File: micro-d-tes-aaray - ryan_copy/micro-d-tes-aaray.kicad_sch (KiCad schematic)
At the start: 23 parts, among them J22 Conn_01x01_Socket, J23 Conn_01x01_Socket, J24 Conn_01x01_Socket, J25 Conn_01x01_Socket, J26 Conn_01x01_Socket, J27 Conn_01x01_Socket, J28 Conn_01x01_Socket, J29 Conn_01x01_Socket, J30 Conn_01x01_Socket, J31 Conn_01x01_Socket, J32 Conn_01x01_Socket, J33 Conn_01x01_Socket, J34 Conn_01x01_Socket, J35 Conn_01x01_Socket, J36 Conn_01x01_Socket, J37 Conn_01x01_Socket, J38 Conn_01x01_Socket, J39 Conn_01x01_Socket, J40 Conn_01x01_Socket, J41 Conn_01x01_Socket, J42 DB25_Plug

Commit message: update
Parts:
- H3, H4: footprint 0_footprint_Library:MountingHole_3mm_4-40_DIN965_Pad -> 0_footprint_Library:MountingHole_3mm_2-56_DIN965_Pad
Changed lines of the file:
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@@
       (effects (font (size 1.27 1.27)) (justify left))
     )
-    (property "Footprint" "0_footprint_Library:MountingHole_3mm_4-40_DIN965_Pad" (at 55.88 143.51 0)
+    (property "Footprint" "0_footprint_Library:MountingHole_3mm_2-56_DIN965_Pad" (at 55.88 143.51 0)
       (effects (font (size 1.27 1.27)) hide)
     )
@@
       (effects (font (size 1.27 1.27)) (justify left))
     )
-    (property "Footprint" "0_footprint_Library:MountingHole_3mm_4-40_DIN965_Pad" (at 59.69 143.51 0)
-      (effects (font (size 1.27 1.27)) hide)
-    )
+    (property "Footprint" "0_footprint_Library:MountingHole_3mm_2-56_DIN965_Pad" (at 59.69 143.51 0)
+      (effects (font (size 1.27 1.27)) hide)
+    )

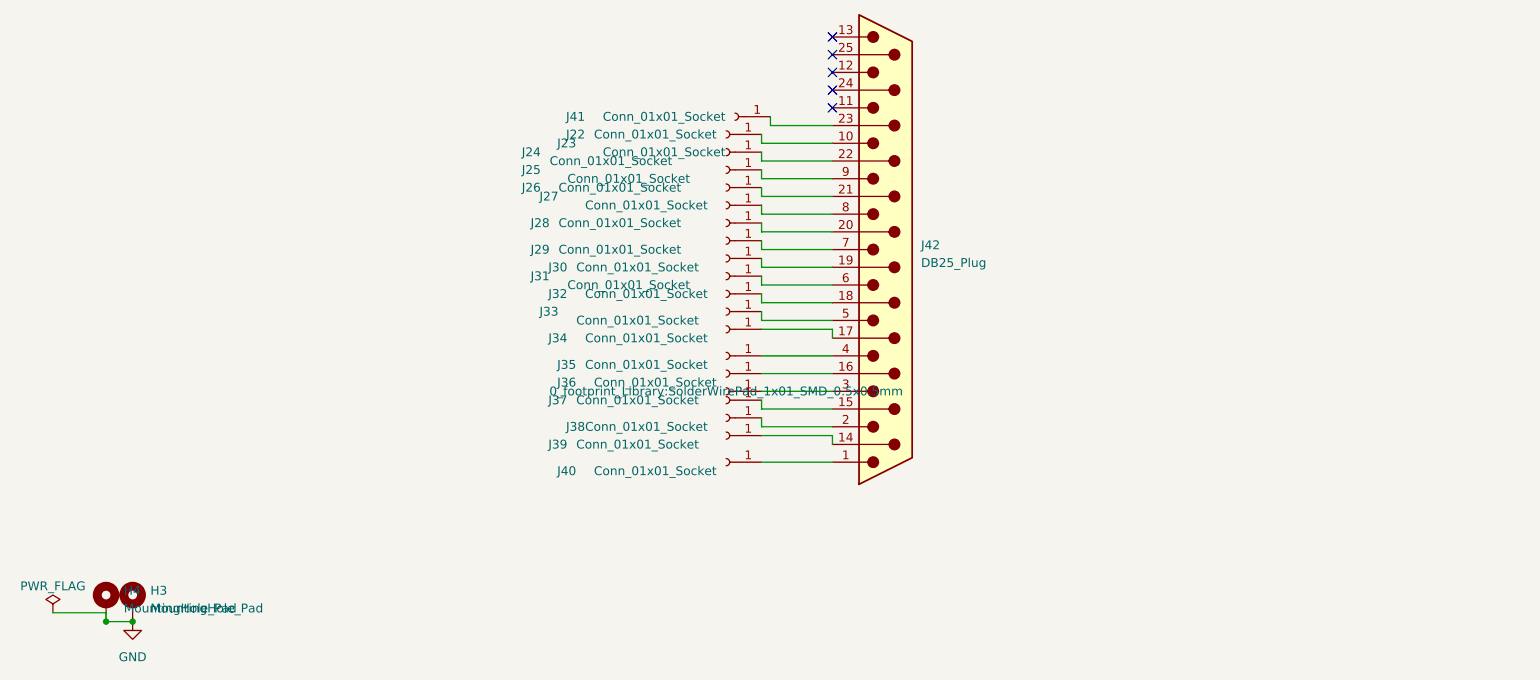
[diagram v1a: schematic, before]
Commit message: Update
finished old cad design
made new cad design
maybe finalized PCB layout
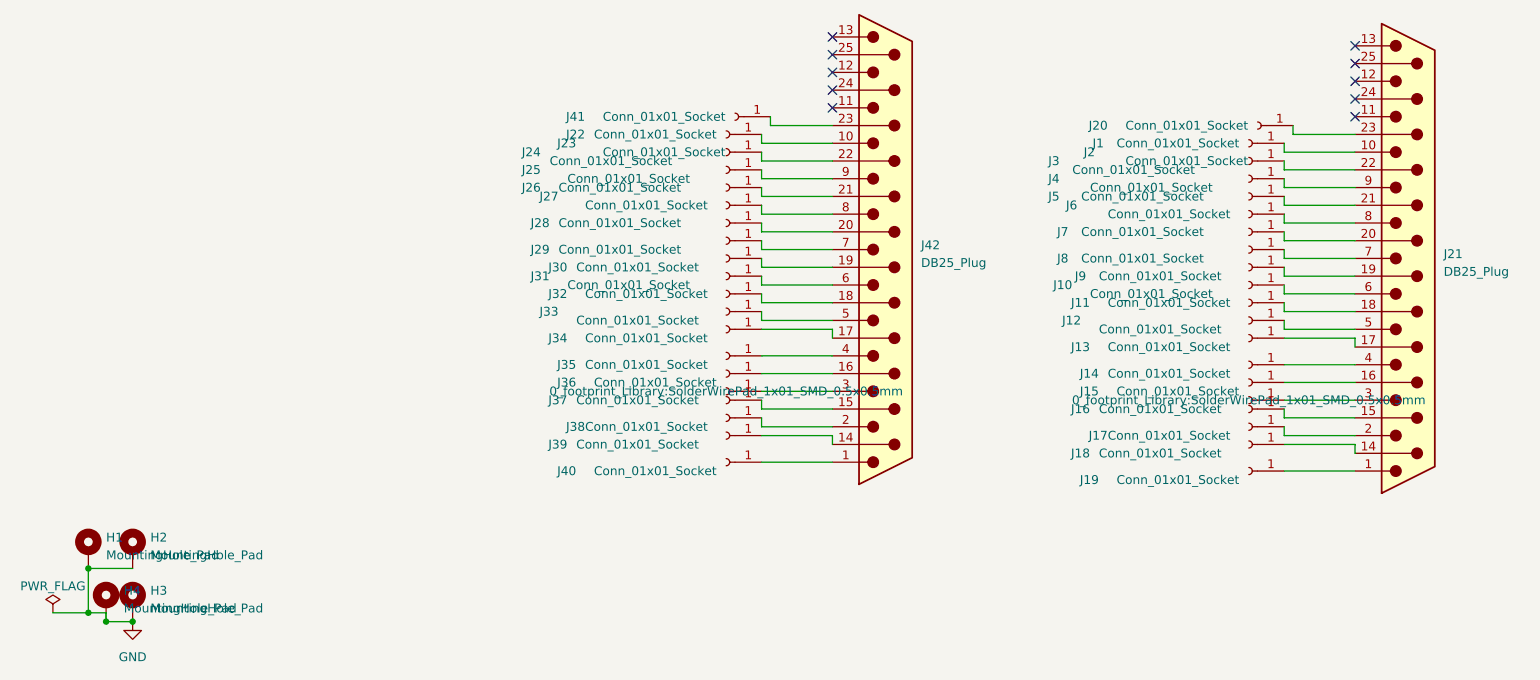
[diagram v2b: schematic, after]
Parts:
- added H1, H2: MountingHole_Pad, 0_footprint_Library:MountingHole_3mm_2-56_DIN965_Pad, symbol Mechanical:MountingHole_Pad
- added J1, J10, J11, J12, J13, J14, J15, J16, J17, J18, J19, J2, J20, J3, J4, J5, J6, J7, J8, J9: Conn_01x01_Socket, 0_footprint_Library:SolderWirePad_1x01_SMD_0.5x0.5mm, symbol Connector:Conn_01x01_Socket
- added J21: DB25_Plug, 0_footprint_Library:Norcomp-380-025-113L001-microd_Updated, symbol Connector:DB25_Plug
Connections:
- net GND: now also H1.1, H2.1
- new net: J13.1 (Pin_1), J21.4
- new net: J2.1 (Pin_1), J21.22 (P22)
- new net: J21.19 (P19), J8.1 (Pin_1)
- new net: J21.9, J3.1 (Pin_1)
- new net: J11.1 (Pin_1), J21.5
- new net: J21.7, J7.1 (Pin_1)
- new net: J21.6, J9.1 (Pin_1)
- new net: J14.1 (Pin_1), J21.16 (P16)
- new net: J16.1 (Pin_1), J21.15 (P15)
- new net: J1.1 (Pin_1), J21.10
- new net: J18.1 (Pin_1), J21.14 (P14)
- new net: J15.1 (Pin_1), J21.3
- new net: J19.1 (Pin_1), J21.1
- new net: J12.1 (Pin_1), J21.17 (P17)
- new net: J10.1 (Pin_1), J21.18 (P18)
- new net: J17.1 (Pin_1), J21.2
- new net: J21.20 (P20), J6.1 (Pin_1)
- new net: J21.21 (P21), J4.1 (Pin_1)
- new net: J20.1 (Pin_1), J21.23 (P23)
- new net: J21.8, J5.1 (Pin_1)
- no-connect marks 5 -> 10
